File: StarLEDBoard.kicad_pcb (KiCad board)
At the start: 2 copper layers, 20 x 21.4 mm, 8 parts

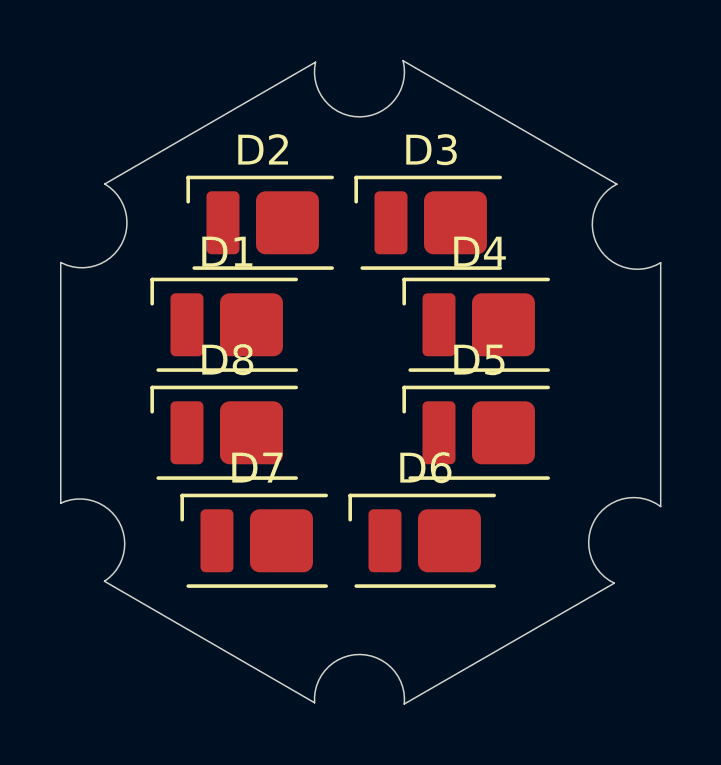
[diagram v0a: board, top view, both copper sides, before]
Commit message: Ordered Board
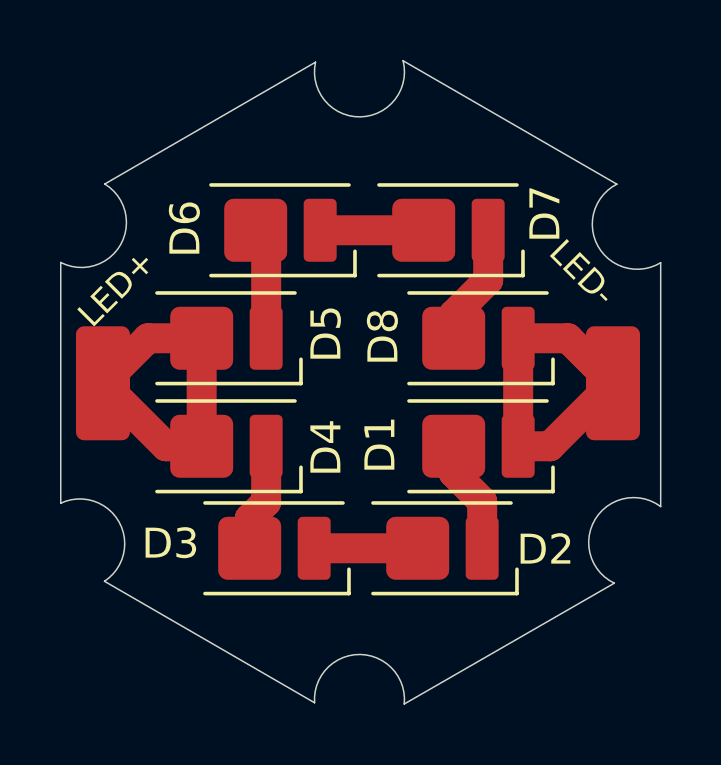
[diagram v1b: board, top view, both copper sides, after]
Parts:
- added J1: Conn_01x02_Socket, Library:LEDConnector, F.Cu at (128.8, 93.3)
- moved D2 12.4 mm to (140.2, 98.8), turned to 180 degrees
- moved D7 12.1 mm to (140.3, 88.2), turned to 180 degrees
- moved D3 12.0 mm to (134.6, 98.8), turned to 180 degrees
- moved D6 11.4 mm to (134.8, 88.2), turned to 180 degrees
- moved D4 9.36 mm to (132.9, 95.4), turned to 180 degrees
- moved D1 9.29 mm to (141.3, 95.4), turned to 180 degrees
- moved D5 9.01 mm to (132.9, 91.9), turned to 180 degrees
- moved D8 8.93 mm to (141.3, 91.9), turned to 180 degrees
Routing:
- net /LED+: track 0.00 -> 11.7 mm
- net /LED-: track 0.00 -> 11.4 mm
- net Net-(D7-K): track 0.00 -> 4.08 mm
- net Net-(D1-A): track 0.00 -> 3.79 mm
- net Net-(D5-K): track 0.00 -> 3.74 mm
- net Net-(D3-A): track 0.00 -> 3.63 mm
- net Net-(D6-K): track 0.00 -> 3.45 mm
- net Net-(D2-A): track 0.00 -> 3.45 mm
